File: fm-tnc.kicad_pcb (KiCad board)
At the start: 2 copper layers, 99.1 x 68.6 mm, 105 parts, among them IC11 LM2936-3.0_TO92, IC12 LM2936-3.0, IC31 BK4802P, IC32 NM(PIC12LF1501-IP), J11 Conn_01x03, J12 Conn_01x06_Female, J13 Conn_01x09_Female, J14 Conn_01x04_Male, J15 Conn_01x05_Male, J16 Conn_01x06_Female, J17 Conn_01x08_Female, J18 USB_C_POW, J31 NM, J32 Conn_01x06_Male, J81 Conn_Coaxial, Q11 NM(DTC114E), X31 Crystal

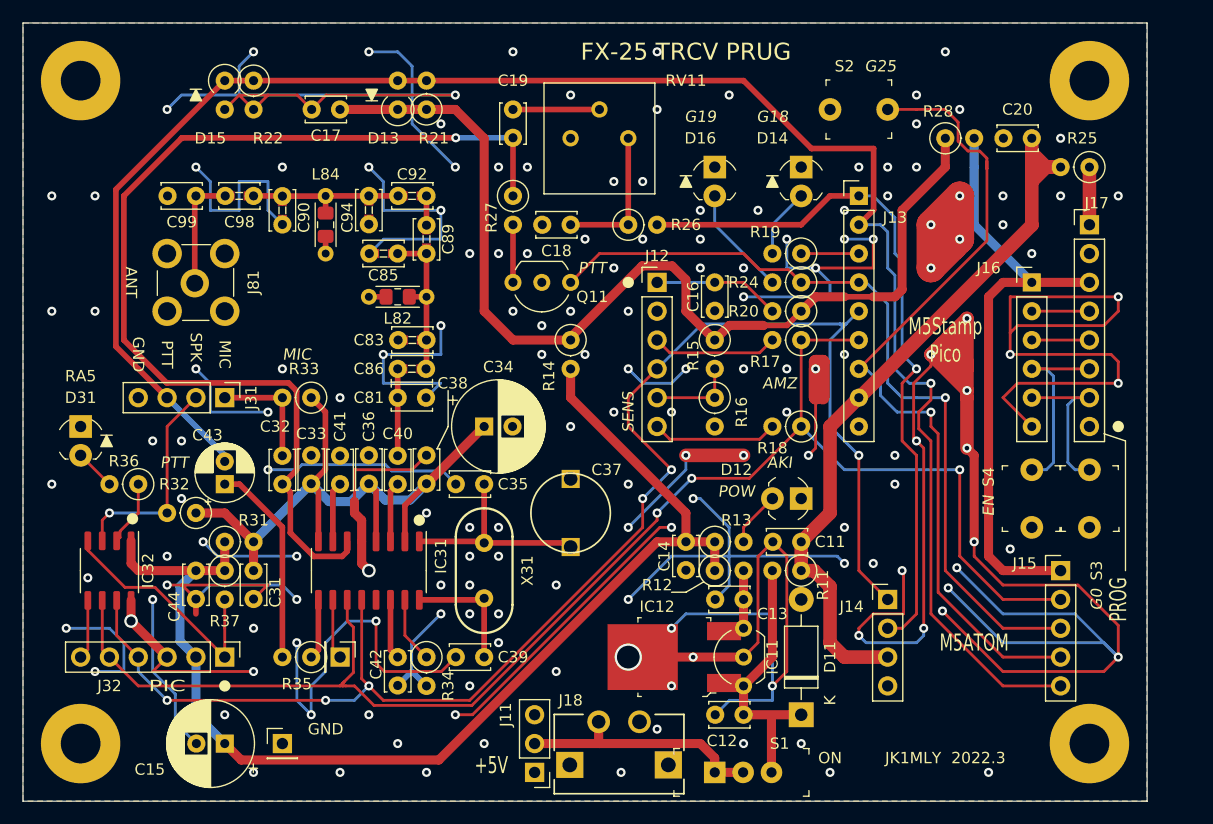
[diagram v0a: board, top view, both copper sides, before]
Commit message: Add files via upload
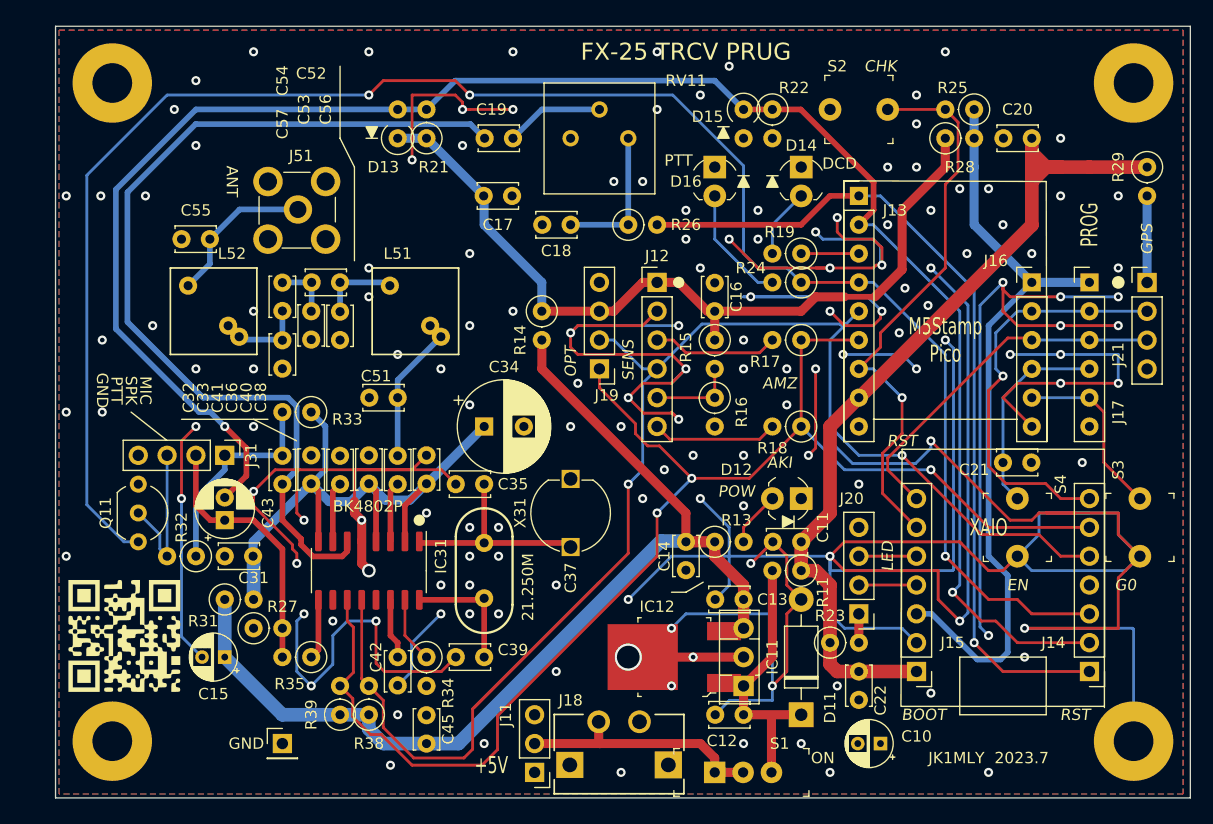
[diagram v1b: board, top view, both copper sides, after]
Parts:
- removed C44: NM, Capacitor_THT:C_Disc_D3.4mm_W2.1mm_P2.50mm
- removed C81, C83, C85, C86, C89, C90, C92, C94, C98, C99: 10p, Capacitor_THT:C_Disc_D3.4mm_W2.1mm_P2.50mm
- removed C82, C84, C87, C88, C91, C93, C95, C97: 1p, digikey-footprints:0603
- removed D31: NM(LED), digikey-footprints:LED_3mm_Radial
- removed IC32: NM(PIC12LF1501-IP), Package_SO:SOP-8_3.9x4.9mm_P1.27mm
- removed J32: Conn_01x06_Male, Connector_PinHeader_2.54mm:PinHeader_1x06_P2.54mm_Vertical
- removed J81: Conn_Coaxial, digikey-footprints:RF_SMA_Vertical_5-1814832-1
- removed L81, L83: 10n, Inductor_SMD:L_0805_2012Metric_Pad1.15x1.40mm_HandSolder
- removed L82, L84: 1u, Resistor_THT:R_Axial_DIN0204_L3.6mm_D1.6mm_P5.08mm_Horizontal
- removed R12, R20: 0, Resistor_THT:R_Axial_DIN0207_L6.3mm_D2.5mm_P2.54mm_Vertical
- removed R36: nM, Resistor_THT:R_Axial_DIN0207_L6.3mm_D2.5mm_P2.54mm_Vertical
- removed R37: NM, Resistor_THT:R_Axial_DIN0207_L6.3mm_D2.5mm_P2.54mm_Vertical
- removed TP31: TestPoint, Connector_PinHeader_2.54mm:PinHeader_1x01_P2.54mm_Vertical
- added ?: , , F.Cu at (50.8, 59.7)
- added ?: , , F.Cu at (68.6, 59.7)
- added C10: 100u, Capacitor_THT:CP_Radial_D4.0mm_P2.00mm, F.Cu at (108.6, 96.5)
- added C21: NM, Capacitor_THT:C_Disc_D3.4mm_W2.1mm_P2.50mm, F.Cu at (119.4, 71.8)
- added C22: 0.1u, Capacitor_THT:C_Disc_D3.4mm_W2.1mm_P2.50mm, F.Cu at (106.7, 90.2)
- added C45: 0.1u, Capacitor_THT:C_Disc_D3.4mm_W2.1mm_P2.50mm, F.Cu at (68.6, 96.5)
- added C51: 10p, Capacitor_THT:C_Disc_D3.4mm_W2.1mm_P2.50mm, F.Cu at (66.0, 66.0)
- added C52: 22p, Capacitor_THT:C_Disc_D3.4mm_W2.1mm_P2.50mm, F.Cu at (61.0, 55.9)
- added C53: 18p, Capacitor_THT:C_Disc_D3.4mm_W2.1mm_P2.50mm, F.Cu at (58.4, 60.9)
- added C54: 22p, Capacitor_THT:C_Disc_D3.4mm_W2.1mm_P2.50mm, F.Cu at (55.9, 55.9)
- added C55: 10p, Capacitor_THT:C_Disc_D3.4mm_W2.1mm_P2.50mm, F.Cu at (49.5, 52.1)
- added C56: NM, Capacitor_THT:C_Disc_D3.4mm_W2.1mm_P2.50mm, F.Cu at (61.0, 58.5)
- added C57: NM, Capacitor_THT:C_Disc_D3.4mm_W2.1mm_P2.50mm, F.Cu at (55.9, 61.0)
- added G***: LOGO, LOGO, F.Cu at (41.9, 87.0)
- added J19: Conn_01x04_Socket, Connector_PinHeader_2.54mm:PinHeader_1x04_P2.54mm_Vertical, F.Cu at (83.8, 63.5)
- added J20: Conn_01x04_Socket, Connector_PinHeader_2.54mm:PinHeader_1x04_P2.54mm_Vertical, F.Cu at (106.7, 85.1)
- added J21: Conn_01x04_Socket, Connector_PinHeader_2.54mm:PinHeader_1x04_P2.54mm_Vertical, F.Cu at (132.1, 55.9)
- added J51: Conn_Coaxial, digikey-footprints:RF_SMA_Vertical_5-1814832-1, F.Cu at (57.1, 49.5)
- added L51: 20n, usr-Library:coil3_7mm, F.Cu at (67.6, 58.4)
- added L52: 20n, usr-Library:coil3_7mm, F.Cu at (49.8, 58.4)
- added R23: NM, Resistor_THT:R_Axial_DIN0207_L6.3mm_D2.5mm_P2.54mm_Vertical, F.Cu at (104.1, 87.6)
- added R29: NM, Resistor_THT:R_Axial_DIN0207_L6.3mm_D2.5mm_P2.54mm_Vertical, F.Cu at (132.1, 45.7)
- added R38: 3.3k, Resistor_THT:R_Axial_DIN0207_L6.3mm_D2.5mm_P2.54mm_Vertical, F.Cu at (63.5, 94.0)
- added R39: 3.3k, Resistor_THT:R_Axial_DIN0207_L6.3mm_D2.5mm_P2.54mm_Vertical, F.Cu at (61.0, 94.0)
- C15: footprint Capacitor_THT:CP_Radial_D7.5mm_P2.50mm -> Capacitor_THT:CP_Radial_D4.0mm_P2.00mm
- C18: value 1000p -> 0.01u
- C19: value 0.1u -> 1u
- C31, C36, C38: value 1u -> 0.1u
- C34: footprint Capacitor_THT:CP_Radial_D8.0mm_P2.50mm -> Capacitor_THT:CP_Radial_D8.0mm_P3.50mm
- C35: value 27p -> 22p
- C39: value 27p -> 33p
- C40: value 100p -> 1000p
- D11: value 1N4002 -> 1N4007
- IC11: value LM2936-3.0_TO92 -> NM(TO220); footprint Package_TO_SOT_THT:TO-92_Inline_Wide -> Package_TO_SOT_THT:TO-126-3_Vertical
- IC12: value LM2936-3.0 -> NJM2845DL1-33
- J14: value Conn_01x04_Male -> Conn_01x07_Socket; footprint Connector_PinHeader_2.54mm:PinHeader_1x04_P2.54mm_Vertical -> Connector_PinHeader_2.54mm:PinHeader_1x07_P2.54mm_Vertical
- J15: value Conn_01x05_Male -> Conn_01x07_Socket; footprint Connector_PinHeader_2.54mm:PinHeader_1x05_P2.54mm_Vertical -> Connector_PinHeader_2.54mm:PinHeader_1x07_P2.54mm_Vertical
- J17: value Conn_01x08_Female -> Conn_01x06_Female; footprint Connector_PinHeader_2.54mm:PinHeader_1x08_P2.54mm_Vertical -> UserLib:PinHeader_1x06_P2.54mm_Vertical
- Q11: value NM(DTC114E) -> NM(DTC143E)
- R25: value NM -> 10k
- R26: value 10k -> 4.7k
- R34: value 10k -> NM
- S2, S3, S4: footprint UserLib:Switch_2P -> usr-Library:Switch_2P
- X31: value Crystal -> 21.250
- moved D15 45.8 mm to (96.5, 40.6)
- moved R22 45.8 mm to (99.1, 40.6)
- moved R27 44.4 mm to (53.3, 86.4), turned to 0 degrees
- moved Q11 42.0 mm to (43.2, 73.7), turned to -90 degrees
- moved J14 18.9 mm to (127.0, 90.2), turned to 180 degrees
- moved J15 15.5 mm to (111.8, 90.2), turned to 180 degrees
- moved C17 14.8 mm to (73.6, 48.3), turned to 0 degrees
- moved R25 11.4 mm to (116.8, 40.6)
- moved C15 7.62 mm to (50.8, 88.9)
- moved S3 5.12 mm to (131.4, 77.5)
- moved J17 5.08 mm to (127.0, 55.9)
- moved J31 5.08 mm to (50.8, 71.1)
- moved R31 5.08 mm to (50.8, 83.8)
- moved TP3 3.90 mm to (130.9, 38.3)
- moved TP5 3.90 mm to (130.9, 96.3)
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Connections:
- C13 pad 1: /cpu/+3.3V-REG -> +3V3
- C16 pad 1: Net-(C16-Pad1) -> /cpu/LMT_3.3V
- C17 pad 1: /cpu/M5_3.3V -> /cpu/LMT_3.3V
- C40 pad 2: TRXIO -> Net-(C40-Pad2)
- C43 pad 1: Net-(C43-Pad1) -> /trx/SPK
- C43 pad 2: TNC_IN -> M5_ADC
- D13 pad 1: /cpu/M5_3.3V -> /cpu/LMT_3.3V
- D13 pad 2: TNC_IN -> M5_ADC
- D15 pad 1: TNC_IN -> M5_ADC
- IC11 pad 3: /cpu/+3.3V-REG -> +3V3
- IC12 pad 3: /cpu/+3.3V-REG -> +3V3
- IC31 pad 10: Net-(IC31-Pad10) -> unconnected-(IC31-EARON-Pad10)
- J12 pad 1: Net-(C16-Pad1) -> /cpu/LMT_3.3V
- J13 pad 1: /cpu/M5_P26 -> M5_DAC
- J13 pad 2: TNC_IN -> M5_ADC
- J14 pad 1: M5_SDA -> M5_DAC
- J14 pad 2: /cpu/M5_P26 -> M5_ADC
- J14 pad 3: +5V -> /cpu/M5_P19
- J14 pad 4: GND -> unconnected-(J14-Pin_4-Pad4)
- J15 pad 1: Net-(J15-Pad1) -> +5V
- J15 pad 2: M5_SCL -> GND
- J15 pad 3: /cpu/M5_P19 -> Net-(J15-Pin_3)
- J15 pad 4: /cpu/M5_P25 -> Net-(J15-Pin_4)
- J15 pad 5: TNC_IN -> Net-(J15-Pin_5)
- J16 pad 1: Net-(J15-Pad1) -> Net-(J15-Pin_3)
- J17 pad 1: Net-(J17-Pad1) -> Net-(J15-Pin_3)
- J17 pad 2: GND -> /cpu/M5_TXD
- J17 pad 3: Net-(J15-Pad1) -> /cpu/M5_RXD
- J17 pad 4: /cpu/M5_TXD -> /cpu/M5_EN
- J17 pad 5: /cpu/M5_RXD -> /cpu/M5_IO0
- J17 pad 6: /cpu/M5_EN -> GND
- J31 pad 2: /trx/PTT -> /trx/SPK
- J31 pad 3: TNC_IN -> TNC_PTT
- Q11 pad 1: /cpu/M5_P19 -> GND
- Q11 pad 2: GND -> TNC_PTT
- Q11 pad 3: Net-(Q11-Pad3) -> /cpu/M5_P19
- R14 pad 1: /cpu/M5_3.3V -> /cpu/LMT_3.3V
- R15 pad 1: /cpu/M5_3.3V -> /cpu/LMT_3.3V
- R21 pad 1: /cpu/M5_3.3V -> /cpu/LMT_3.3V
- R21 pad 2: TNC_IN -> M5_ADC
- R22 pad 1: TNC_IN -> M5_ADC
- R25 pad 1: Net-(J17-Pad1) -> Net-(J15-Pin_3)
- R25 pad 2: +5V -> /cpu/M5_P25
- R26 pad 2: /cpu/M5_P26 -> M5_DAC
- R27 pad 1: TNC_OUT -> GND
- R27 pad 2: Net-(Q11-Pad3) -> /trx/SPK
- R28 pad 1: /cpu/M5_3.3V -> /cpu/LMT_3.3V
- R28 pad 2: Net-(J15-Pad1) -> Net-(J15-Pin_3)
- R32 pad 1: /trx/+3.3V-TR -> /trx/MIC
- R32 pad 2: /trx/PTT -> TNC_PTT
- R35 pad 2: Net-(C43-Pad1) -> /trx/SPK
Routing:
- net M5_ADC: track 0.00 -> 163.0 mm, vias 0 -> 2
- net TNC_IN: track 162.0 -> 0.00 mm, vias 1 -> 0
- net /cpu/M5_3.3V: track 95.6 -> 0.00 mm
- net /cpu/M5_P19: track 70.9 -> 161.1 mm, vias 1 -> 3
- net M5_DAC: track 0.00 -> 74.7 mm, vias 0 -> 1
- net /cpu/LMT_3.3V: track 0.00 -> 73.1 mm
- net Net-(J15-Pin_3): track 0.00 -> 67.3 mm
- net /cpu/M5_P26: track 62.6 -> 0.00 mm, vias 1 -> 0
- net GND: track 679.3 -> 617.6 mm, vias 164 -> 149
- net Net-(J15-Pad1): track 54.0 -> 0.00 mm
- net /cpu/M5_TXD: track 5.08 -> 36.7 mm, vias 0 -> 1
- net /cpu/M5_RXD: track 5.08 -> 32.1 mm
- net /trx/SPK: track 0.00 -> 23.2 mm
- net /cpu/M5_P25: track 73.3 -> 50.3 mm
- net Net-(IC32-Pad4): track 21.9 -> 0.00 mm
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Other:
- board size 99.1 x 68.6 mm -> 100 x 68 mm
- board text added: "21.250M"
- board text added: "3V"
- board text added: "5V"
- board text added: "B"
- board text added: "BK4802P"
- board text added: "BOOT"
- board text added: "C"
- board text added: "CHK"
- board text added: "D"
- board text added: "DCD"
- board text added: "E"
- board text added: "G"
- board text added: "GPS"
- board text added: "I"
- board text added: "JK1MLY 2023.7"
- board text added: "LED"
- board text added: "M"
- board text added: "O"
- board text added: "OPT"
- board text added: "P"
- board text added: "RF"
- board text added: "RST"
- board text added: "RX"
- board text added: "S"
- board text added: "SCL"
- board text added: "SDA"
- board text added: "TX"
- board text added: "V"
- board text added: "XAIO"
- board text removed: "G18"
- board text removed: "G19"
- board text removed: "G25"
- board text removed: "JK1MLY 2022.3"
- board text removed: "M5ATOM"
- board text removed: "PIC"
- board text removed: "RA5"
